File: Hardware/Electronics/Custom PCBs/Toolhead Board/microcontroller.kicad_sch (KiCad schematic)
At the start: 35 parts, among them J1 USB C Receptacle, J2 Conn_02x04_Odd_Even, J3 Conn_02x08_Odd_Even, J4 Conn_02x08_Odd_Even, J5 Conn_02x08_Odd_Even, J6 Conn_02x04_Odd_Even, SW1 BOOT, SW2 RESET, U3 RP2040, U4 W25Q128JVS, Y1 12MHz/12pF/50Ω/20ppm

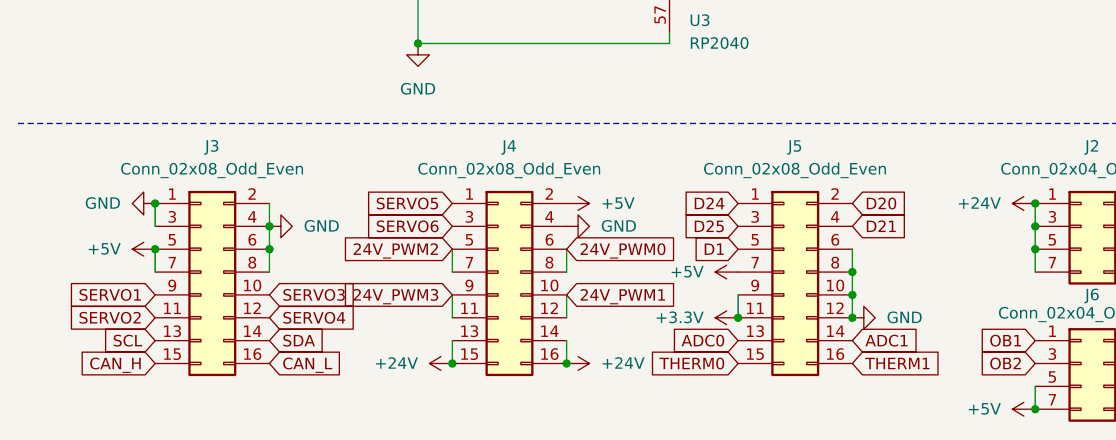
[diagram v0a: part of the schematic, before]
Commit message: Update layout
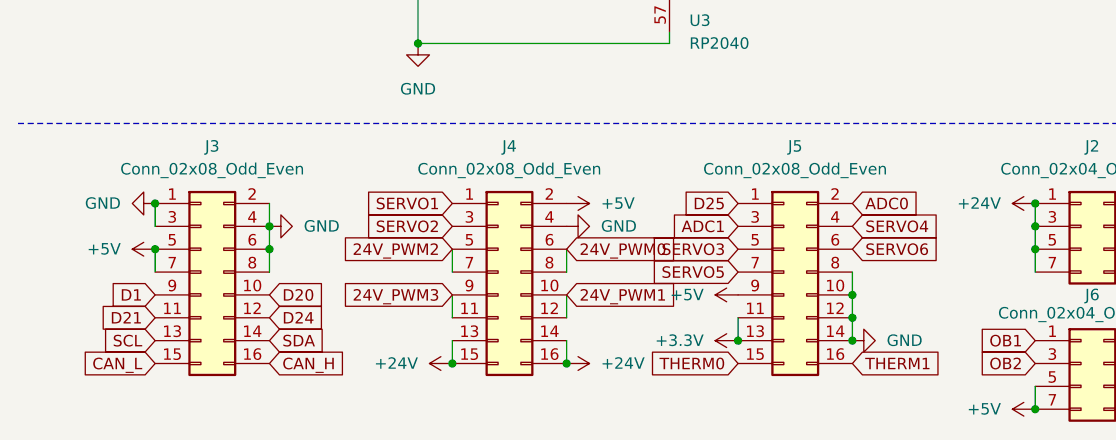
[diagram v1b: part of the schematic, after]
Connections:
- net +3.3V: now also J5.13 (Pin_13); no longer J5.9 (Pin_9)
- net +5V: now also J5.9 (Pin_9); no longer J5.7 (Pin_7)
- net ADC0: now also J5.2 (Pin_2); no longer J5.13 (Pin_13)
- net ADC1: now also J5.3 (Pin_3); no longer J5.14 (Pin_14)
- net CAN_H: now also J3.16 (Pin_16); no longer J3.15 (Pin_15)
- net CAN_L: now also J3.15 (Pin_15); no longer J3.16 (Pin_16)
- net D1: now also J3.9 (Pin_9); no longer J5.5 (Pin_5)
- net D20: now also J3.10 (Pin_10); no longer J5.2 (Pin_2)
- net D21: now also J3.11 (Pin_11); no longer J5.4 (Pin_4)
- net D24: now also J3.12 (Pin_12); no longer J5.1 (Pin_1)
- net D25: now also J5.1 (Pin_1); no longer J5.3 (Pin_3)
- net GND: now also J5.14 (Pin_14); no longer J5.6 (Pin_6)
- net SERVO1: now also J4.1 (Pin_1); no longer J3.9 (Pin_9)
- net SERVO2: now also J4.3 (Pin_3); no longer J3.11 (Pin_11)
- net SERVO3: now also J5.5 (Pin_5); no longer J3.10 (Pin_10)
- net SERVO4: now also J5.4 (Pin_4); no longer J3.12 (Pin_12)
- net SERVO5: now also J5.7 (Pin_7); no longer J4.1 (Pin_1)
- net SERVO6: now also J5.6 (Pin_6); no longer J4.3 (Pin_3)

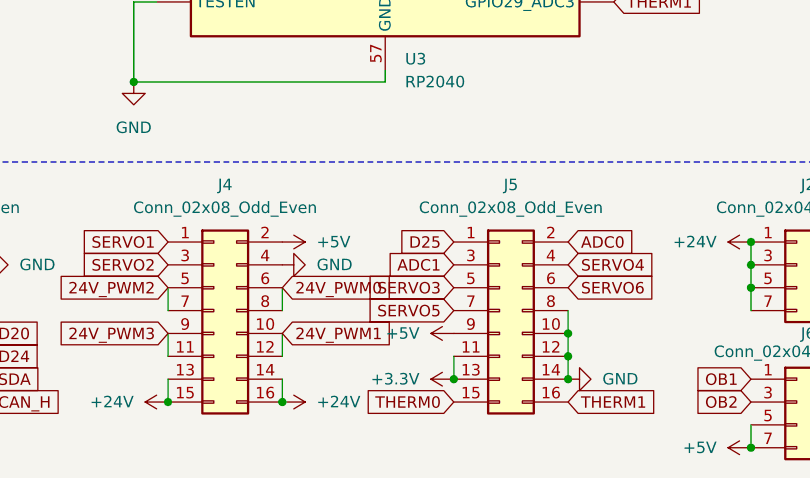
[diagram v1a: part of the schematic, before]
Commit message: Update layout
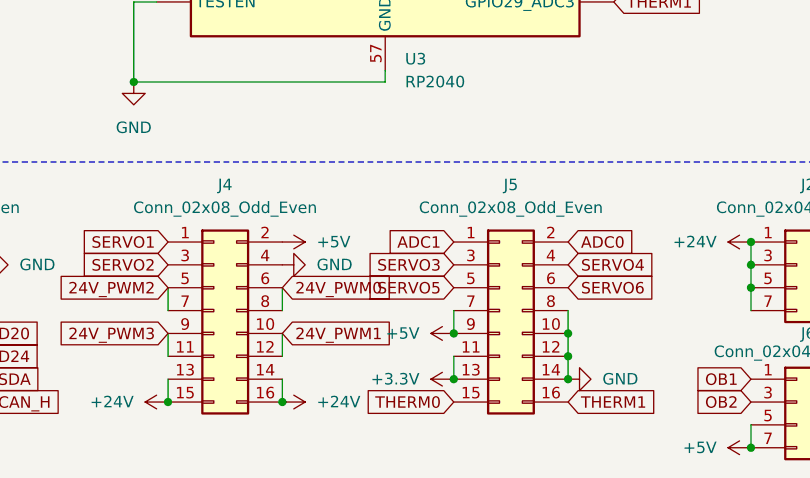
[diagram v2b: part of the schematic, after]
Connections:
- net +5V: now also J5.7 (Pin_7)
- net ADC1: now also J5.1 (Pin_1); no longer J5.3 (Pin_3)
- net D25: no longer J5.1 (Pin_1)
- net SERVO3: now also J5.3 (Pin_3); no longer J5.5 (Pin_5)
- net SERVO5: now also J5.5 (Pin_5); no longer J5.7 (Pin_7)
